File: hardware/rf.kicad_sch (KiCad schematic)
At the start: 6 parts, among them U1 SN74CBT3253, U2 XLV320ADC6120IRTER, Y1 Si5351A-B-GT

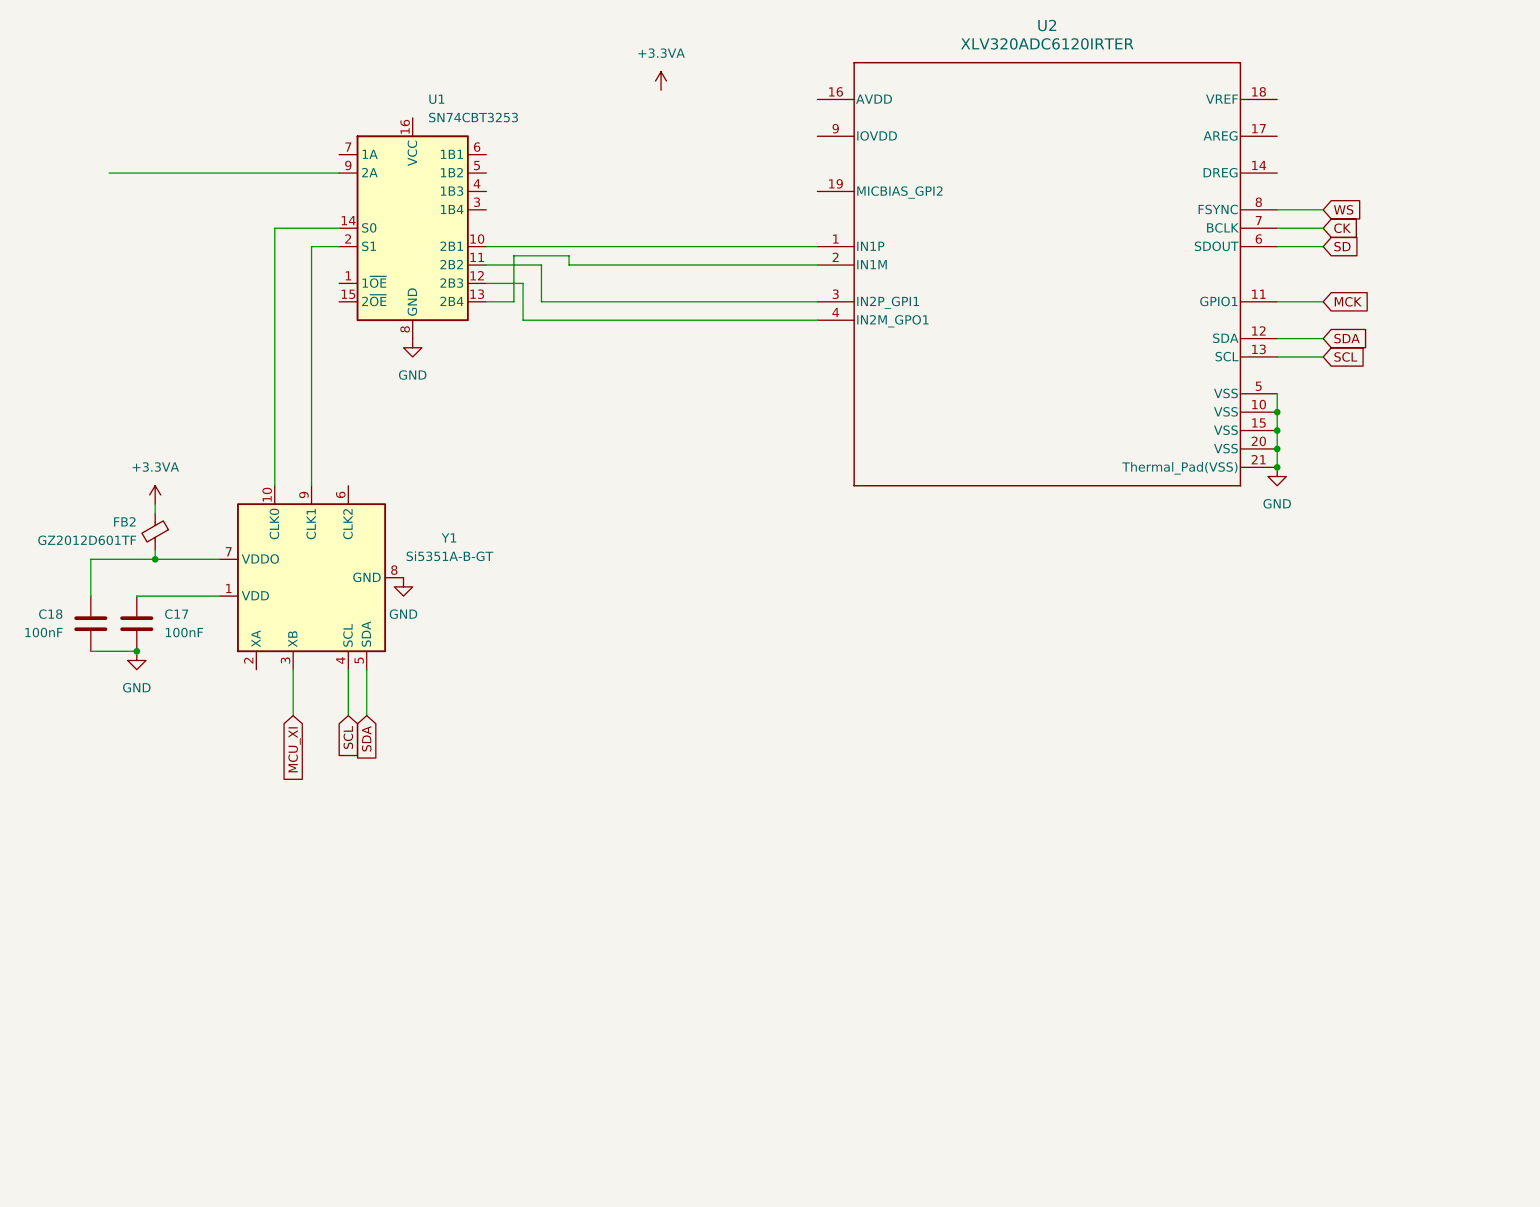
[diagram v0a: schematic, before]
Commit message: amp and audio
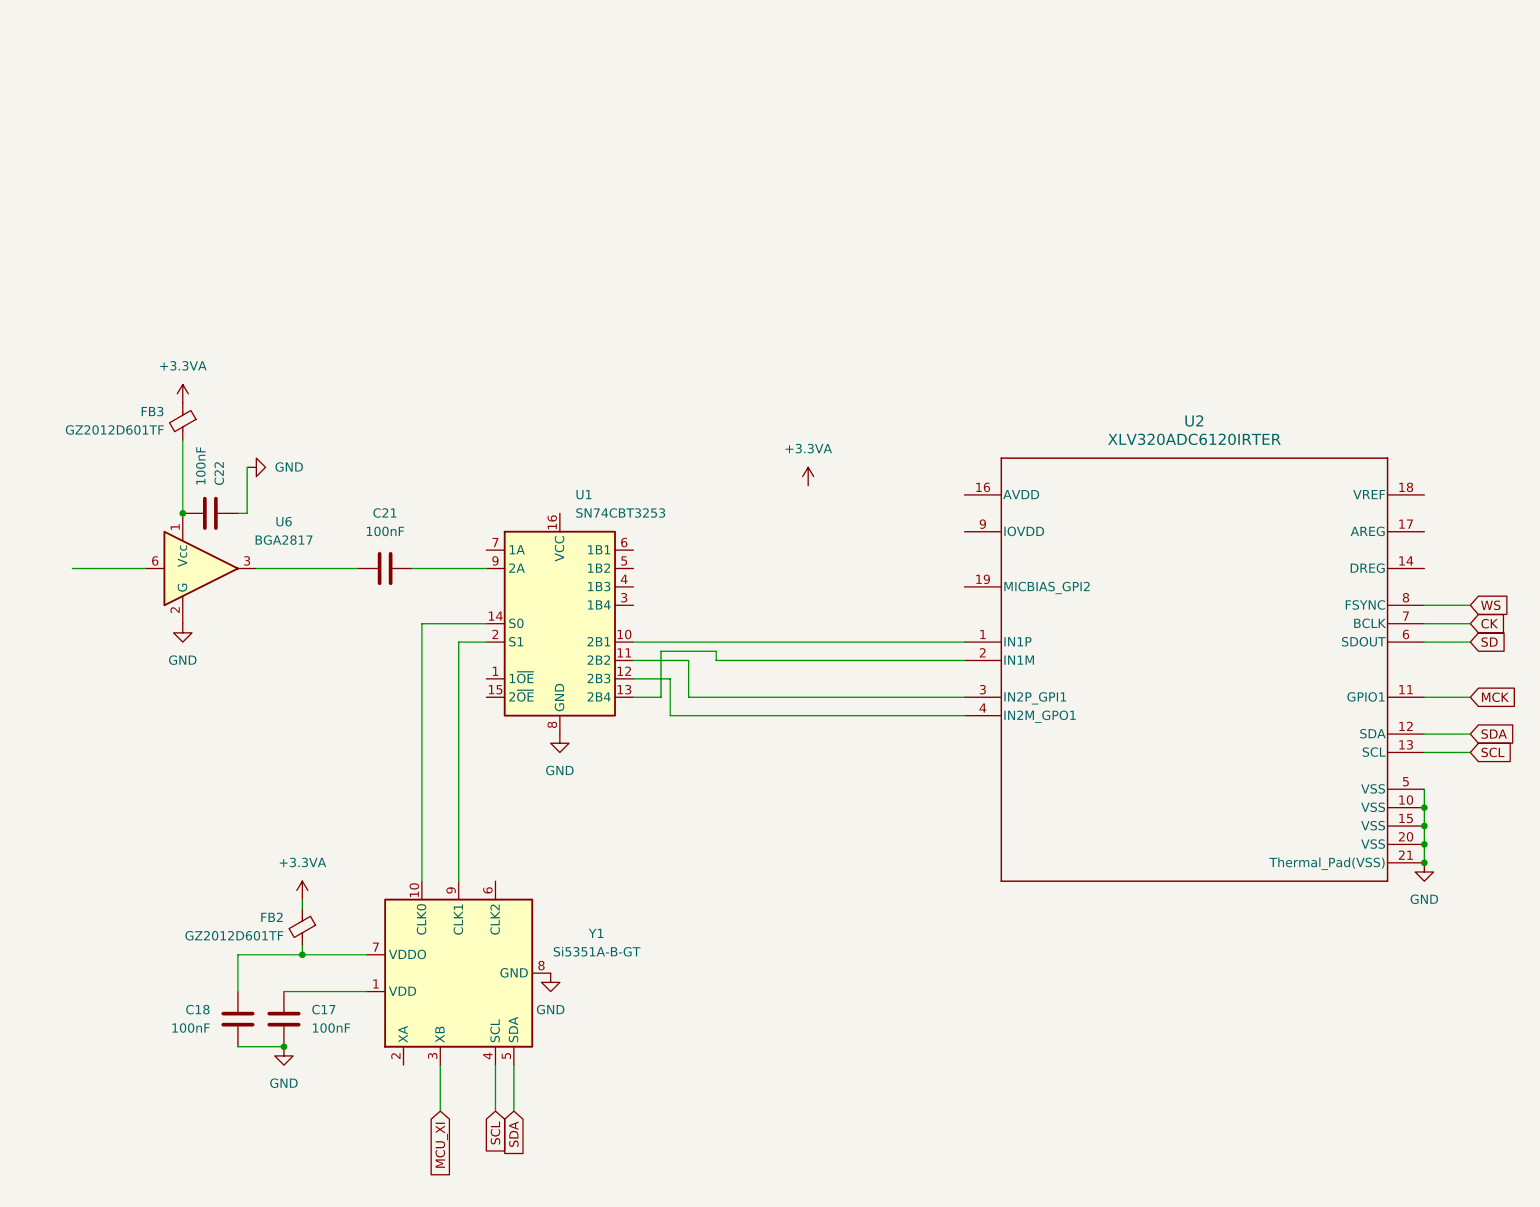
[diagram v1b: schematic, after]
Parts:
- added C21, C22: 100nF, Capacitor_SMD:C_0805_2012Metric_Pad1.18x1.45mm_HandSolder, symbol Device:C
- added FB3: GZ2012D601TF, Inductor_SMD:L_0805_2012Metric_Pad1.05x1.20mm_HandSolder, symbol Device:FerriteBead_Small
- added U6: BGA2817, Package_TO_SOT_SMD:SOT-363_SC-70-6, symbol RF_Amplifier:BGA2817
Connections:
- net +3.3VA: now also FB3.1
- net GND: now also C22.1, U6.2 (G), U6.4 (G), U6.5 (G)
- net at U1.9 (2A): now also C21.1
- new net: C22.2, FB3.2, U6.1 (Vcc)
- new net: C21.2, U6.3
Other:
- moved on the sheet: C17, C18, FB2, U1, U2, Y1
